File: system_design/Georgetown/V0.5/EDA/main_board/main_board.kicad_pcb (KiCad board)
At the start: 2 copper layers, 40.6 x 78.5 mm, 28 parts, among them U1 top_rail_v2, U3 INA219AxD

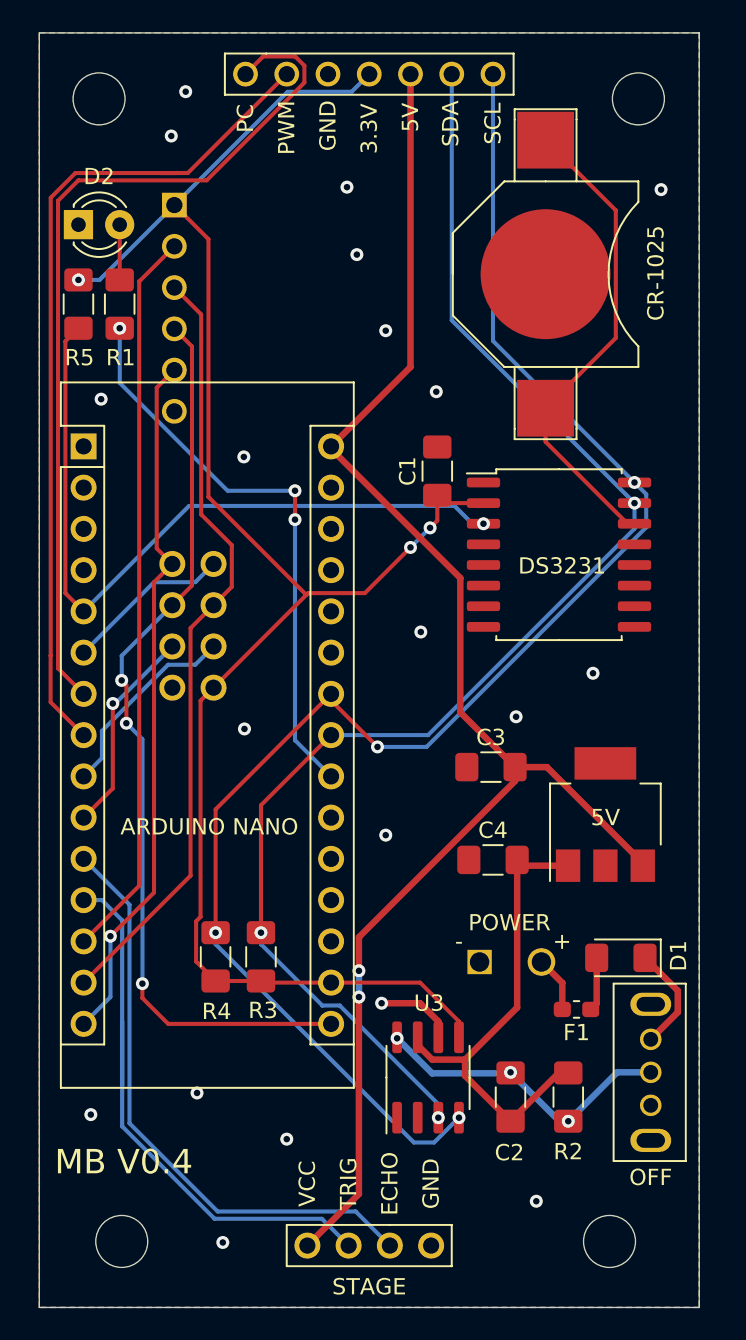
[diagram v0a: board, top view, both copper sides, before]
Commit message: PCB modified
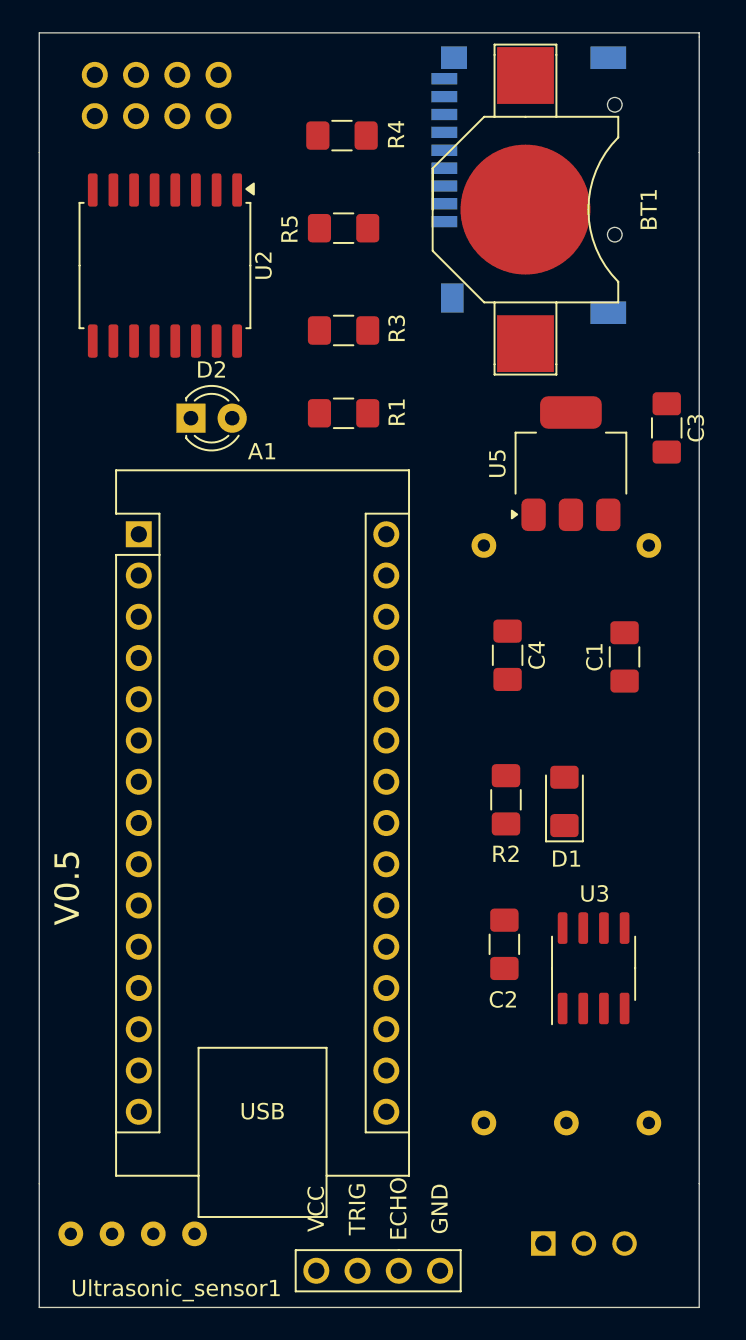
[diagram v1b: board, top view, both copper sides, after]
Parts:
- removed 5V: KA78M05_TO252, Package_TO_SOT_SMD:SOT-223-3_TabPin2
- removed ARDUINO NANO: Arduino_Nano_v2.x-MCU_Module, Module:Arduino_Nano
- removed CR-1025: Battery_Cell, custom:battery_holder_10mm
- removed DS3231: DS3231M, Package_SO:SOIC-16W_7.5x10.3mm_P1.27mm
- removed F1: Fuse, Resistor_SMD:R_0603_1608Metric_Pad1.05x0.95mm_HandSolder
- removed G***: LOGO, UofSC_logo:uofsc_logo_0_75in
- removed MICRO SD: small_microSD, custom:small_microSD_v2
- removed POWER: XP60PW, custom:XT60PW
- removed REF** (x4): MountingHole_3.2mm_M3, MountingHole:MountingHole_3.2mm_M3
- removed STAGE: HCSR04, custom:HCSR04
- removed switch1: grounded_switch, custom:grounded_switch
- added A1: Arduino_Nano_v2.x-MCU_Module, Module:Arduino_Nano, F.Cu at (143.3, 102.2)
- added BT1: Battery_Cell, ARTS-Lab:battery_holder_10mm, F.Cu at (167.1, 82.3)
- added J1: B3B-XH-A_LF__SN_, XH2.54:XH2.54, B.Cu at (170.7, 145.4)
- added P1: SD card socket, ST-TF-003A:SUNTECH_ST-TF-003A, B.Cu at (167.4, 79.5)
- added U2: DS3231M, Package_SO:SOIC-16W_7.5x10.3mm_P1.27mm, F.Cu at (144.9, 85.7)
- added U4: BME280_module, megasaturnv_custom_components:BME280_module, B.Cu at (148.0, 146.6)
- added U5: KA78M05_TO252, Package_TO_SOT_SMD:SOT-223-3_TabPin2, F.Cu at (169.9, 97.9)
- added Ultrasonic_sensor1: HCSR04, ARTS-Lab:HCSR04, F.Cu at (158.0, 146.3)
- U1: value top_rail_v2 -> HX-2S-JH10; footprint custom:top_rail_v2 -> megasaturnv_custom_components:HX-2S-JH10; moved to B.Cu
- moved R4 51.2 mm to (155.8, 77.7), turned to 180 degrees
- moved U1 45.3 mm to (169.6, 120.7), turned to -90 degrees
- moved R3 38.9 mm to (155.9, 89.7), turned to 180 degrees
- moved C3 23.5 mm to (175.8, 95.7), turned to -90 degrees
- moved nRF24L01+1 22.3 mm to (146.9, 85.4), turned to 180 degrees
- moved R2 18.7 mm to (165.9, 118.6)
- moved R5 17.0 mm to (155.9, 83.4), turned to 0 degrees
- moved C1 16.2 mm to (173.2, 109.8)
- moved R1 15.3 mm to (155.9, 94.8), turned to 180 degrees
- moved D2 13.8 mm to (146.5, 95.1)
- moved C4 12.6 mm to (166.0, 109.7), turned to -90 degrees
- moved U3 12.2 mm to (171.3, 129.0)
- moved D1 10.2 mm to (169.5, 118.7), turned to 90 degrees
- moved C2 9.41 mm to (165.8, 127.5)
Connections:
- C1 pad 1: Net-(A1-Pad17) -> Net-(A1-3V3)
- C2 pad 1: Net-(C2-Pad1) -> Net-(D1-K)
- C3 pad 2: Net-(A1-Pad30) -> Net-(A1-VIN)
- D1 pad 1: Net-(D1-Pad1) -> Net-(D1-K)
- D1 pad 2: Net-(D1-Pad2) -> Net-(D1-A)
- R2 pad 1: Net-(C2-Pad1) -> Net-(D1-K)
- R3 pad 1: Net-(A1-Pad17) -> Net-(A1-3V3)
- R3 pad 2: Net-(A1-Pad23) -> Net-(A1-A4)
- R4 pad 1: Net-(A1-Pad17) -> Net-(A1-3V3)
- R4 pad 2: Net-(A1-Pad24) -> Net-(A1-A5)
- R5 pad 2: Net-(A1-Pad17) -> Net-(A1-3V3)
- U1 pad 2: Net-(A1-Pad24) -> Net-(D1-A)
- U1 pad 3: Net-(A1-Pad23) -> unconnected-(U1-B--Pad3)
- U1 pad 4: Net-(A1-Pad30) -> unconnected-(U1-BM-Pad4)
- U1 pad 5: Net-(A1-Pad17) -> unconnected-(U1-B+-Pad5)
- U3 pad 1: Net-(U3-Pad1) -> unconnected-(U3-A1-Pad1)
- U3 pad 2: Net-(U3-Pad2) -> unconnected-(U3-A0-Pad2)
- U3 pad 3: Net-(A1-Pad23) -> Net-(A1-A4)
- U3 pad 4: Net-(A1-Pad24) -> Net-(A1-A5)
- U3 pad 5: Net-(A1-Pad17) -> Net-(A1-3V3)
- U3 pad 8: Net-(C2-Pad1) -> Net-(D1-K)
- nRF24L01+1 pad 1: Net-(A1-Pad17) -> Net-(A1-3V3)
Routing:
- net Net-(A1-Pad17): track 109.2 -> 0.00 mm, vias 3 -> 0
- net Net-(A1-Pad24): track 97.5 -> 0.00 mm, vias 4 -> 0
- net Net-(A1-Pad30): track 94.6 -> 0.00 mm, vias 2 -> 0
- net Net-(A1-Pad23): track 87.2 -> 0.00 mm, vias 3 -> 0
- net Net-(A1-D13): track 56.3 -> 0.00 mm, vias 3 -> 0
- net Net-(A1-Pad7): track 54.6 -> 0.00 mm
- net Net-(A1-Pad8): track 52.6 -> 0.00 mm
- net Net-(A1-D11): track 48.0 -> 0.00 mm
- net Net-(A1-D2): track 46.0 -> 0.00 mm, vias 1 -> 0
- net Net-(A1-Pad13): track 45.1 -> 0.00 mm
- net Net-(A1-D12): track 43.4 -> 0.00 mm, vias 1 -> 0
- net Net-(A1-Pad11): track 36.6 -> 0.00 mm
- net Net-(A1-Pad12): track 36.6 -> 0.00 mm
- net Net-(A1-A3): track 35.4 -> 0.00 mm, vias 3 -> 0
- net Net-(U3-IN-): track 30.4 -> 0.00 mm
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- removed copper zone on B.Cu, net GND
- removed copper zone on F.Cu, net GND
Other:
- board text added: "V0.5"
- board text removed: "MB V0.4"
- board text removed: "OFF"
